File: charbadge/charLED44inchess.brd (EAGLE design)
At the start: 113.9 x 113.9 mm, 7 parts, among them U1 ATTINY85-20P

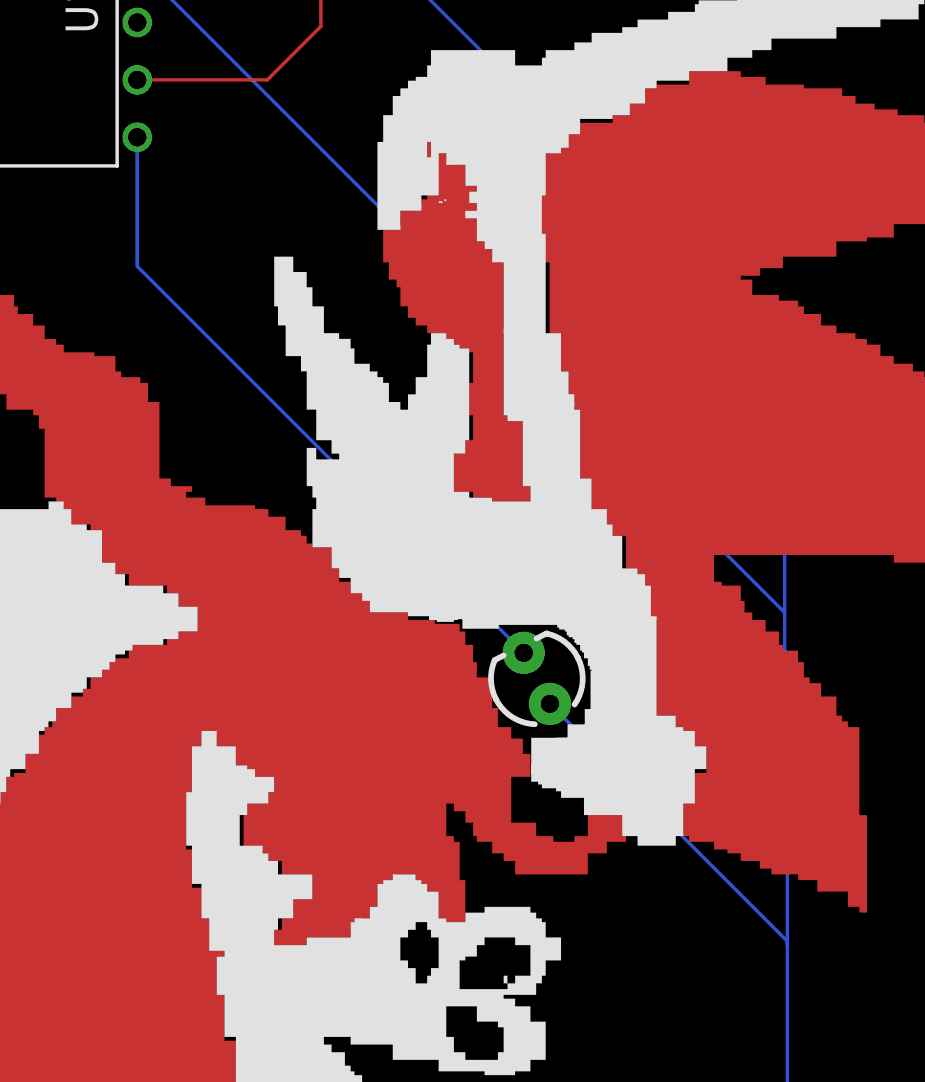
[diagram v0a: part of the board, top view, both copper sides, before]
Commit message: badges
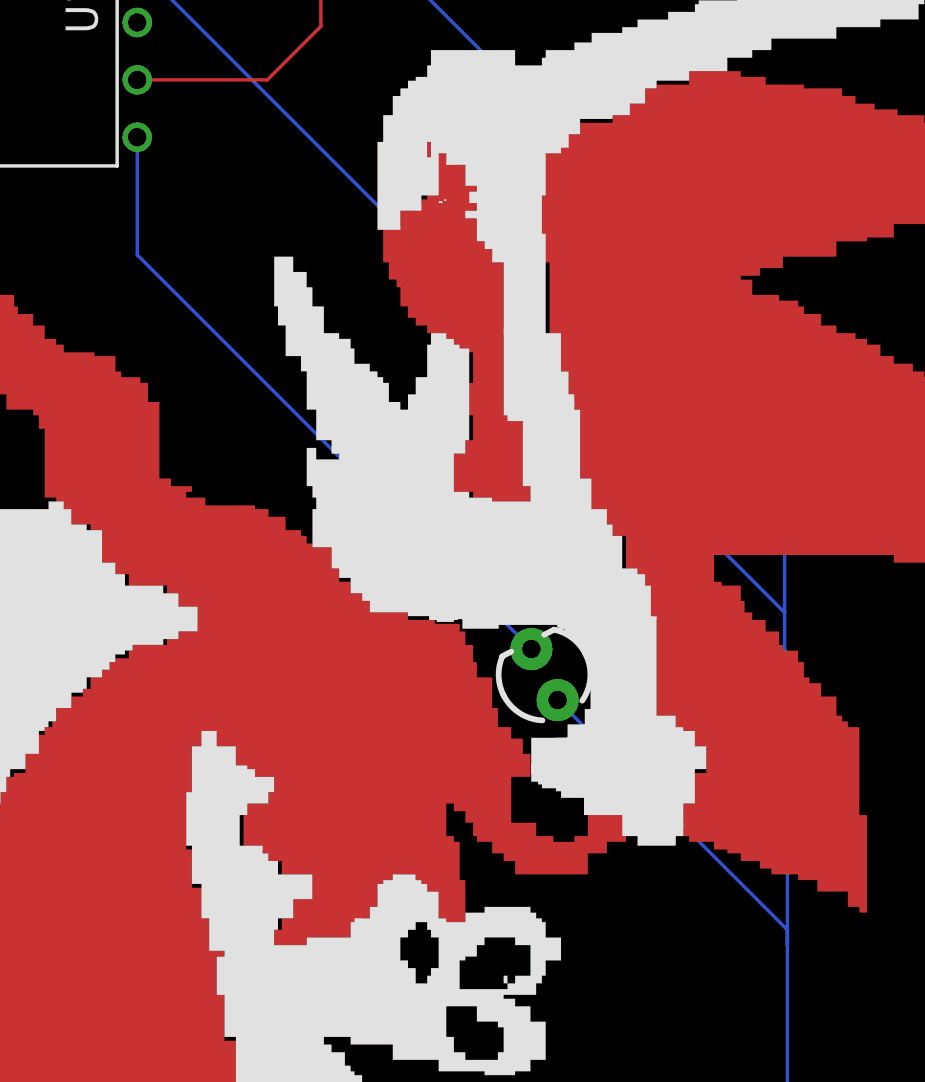
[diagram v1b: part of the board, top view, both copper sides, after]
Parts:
- moved D1 0.38 mm to (74.8, 54.5)
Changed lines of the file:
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@@
 <attribute name="SF_SKU" value="PRT-00783" x="51.977465625" y="9.90615" size="1.778" layer="28" rot="MR180" display="off"/>
 </element>
-<element name="D1" library="SparkFun-LED" library_urn="urn:adsk.eagle:library:529" package="LED_3MM" package3d_urn="urn:adsk.eagle:package:39361/1" value="" x="74.49515" y="54.354115625" rot="MR62.8">
-<attribute name="PROD_ID" value="DIO-08794" x="74.49515" y="54.354115625" size="1.778" layer="28" rot="MR62.8" display="off"/>
+<element name="D1" library="SparkFun-LED" library_urn="urn:adsk.eagle:library:529" package="LED_3MM" package3d_urn="urn:adsk.eagle:package:39361/1" value="" x="74.83378125" y="54.52343125" rot="MR62.8">
+<attribute name="PROD_ID" value="DIO-08794" x="74.83378125" y="54.52343125" size="1.778" layer="28" rot="MR62.8" display="off"/>
 </element>
 <element name="LED1" library="adafruit" package="LED5MM" value="" x="11.763678125" y="45.1254875" rot="R270"/>
@@
 <contactref element="U1" pad="5"/>
 <contactref element="D1" pad="K"/>
-<wire x1="56.803621875" y1="78.311253125" x2="56.803621875" y2="72.5946875" width="0.1524" layer="16"/>
-<wire x1="56.803621875" y1="72.5946875" x2="73.9146375" y2="55.483671875" width="0.1524" layer="16"/>
+<wire x1="56.803621875" y1="78.311253125" x2="56.803621875" y2="73.102634375" width="0.1524" layer="16"/>
+<wire x1="56.803621875" y1="73.102634375" x2="74.25326875" y2="55.6529875" width="0.1524" layer="16"/>
 </signal>
 <signal name="N$6">
@@
 <contactref element="D1" pad="A"/>
 <wire x1="85.586265625" y1="26.58623125" x2="85.586265625" y2="42.583075" width="0.1524" layer="16"/>
-<wire x1="85.586265625" y1="42.583075" x2="85.586265625" y2="42.71395625" width="0.1524" layer="16"/>
-<wire x1="85.586265625" y1="42.71395625" x2="75.075665625" y2="53.22455625" width="0.1524" layer="16"/>
+<wire x1="85.586265625" y1="42.583075" x2="85.586265625" y2="43.221903125" width="0.1524" layer="16"/>
+<wire x1="85.586265625" y1="43.221903125" x2="75.414296875" y2="53.393871875" width="0.1524" layer="16"/>
 <wire x1="85.586265625" y1="42.583075" x2="85.586265625" y2="55.455446875" width="0.1524" layer="16"/>
 <wire x1="85.586265625" y1="55.455446875" x2="85.463028125" y2="55.578684375" width="0.1524" layer="16"/>
